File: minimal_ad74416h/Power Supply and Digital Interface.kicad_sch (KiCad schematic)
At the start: 91 parts, among them T1 ZA9644-AED, U1 MAX17570FATA+, U4 ADP1031ACPZ-2-R7, U5 ADUM1252AUA+, U6 ADUM1252AUA+, U7 ADUM1252AUA+, U8 ADUM1252AUA+

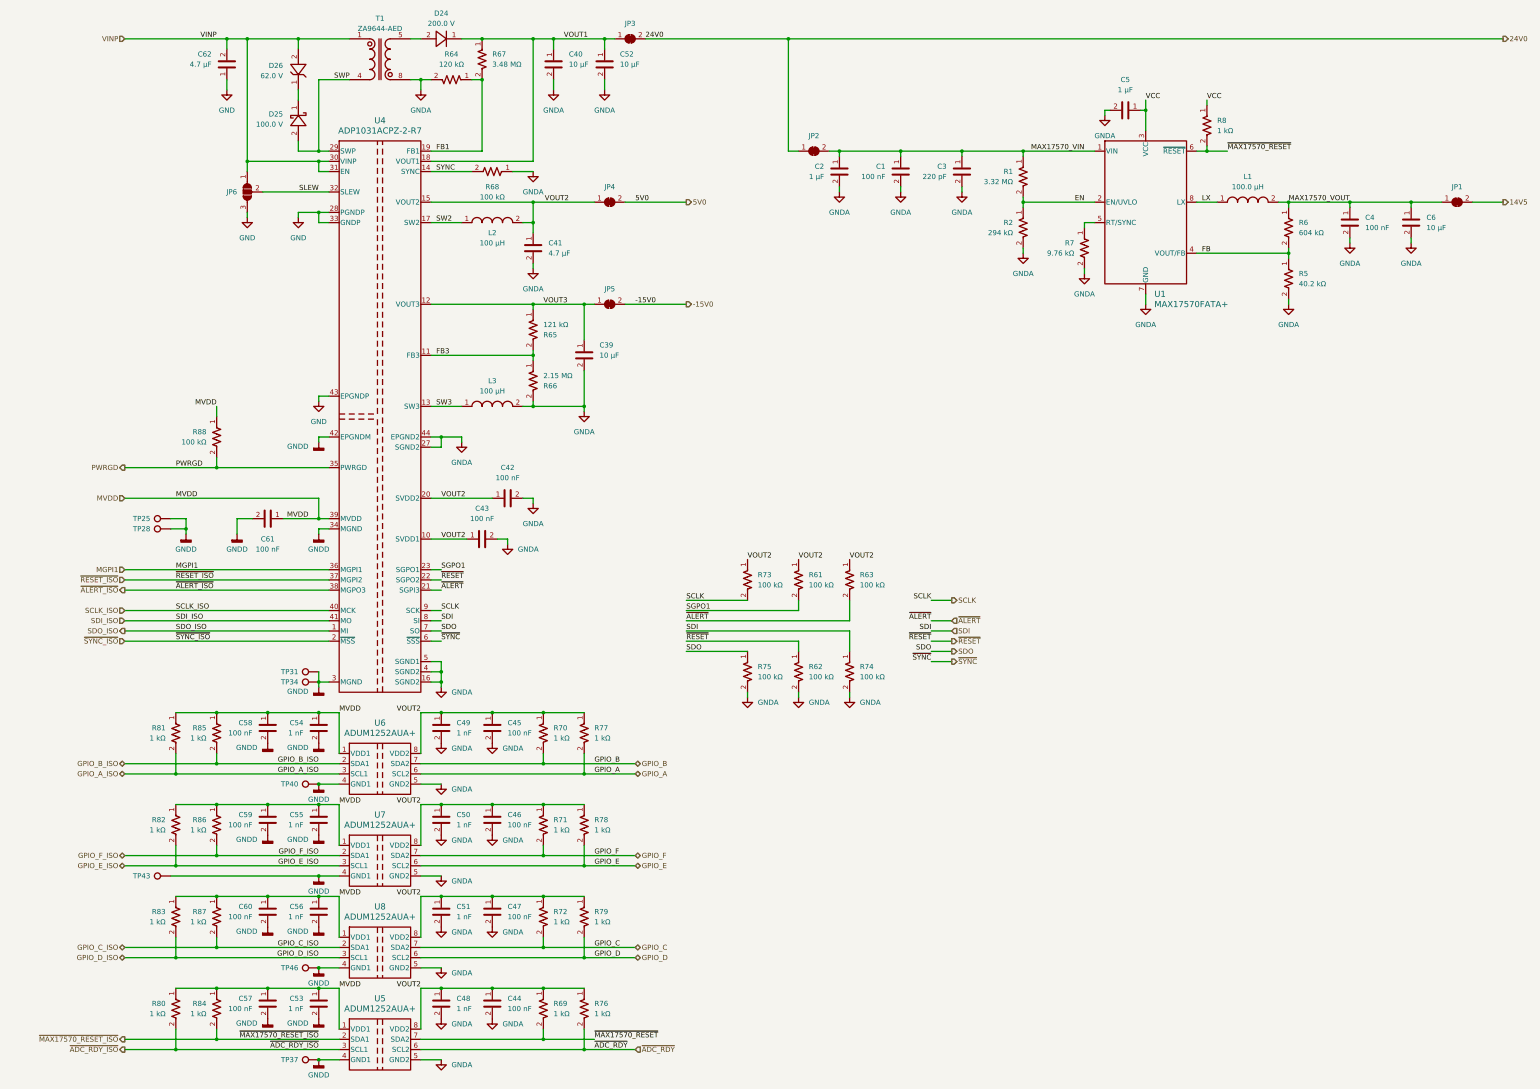
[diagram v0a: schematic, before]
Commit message: backup
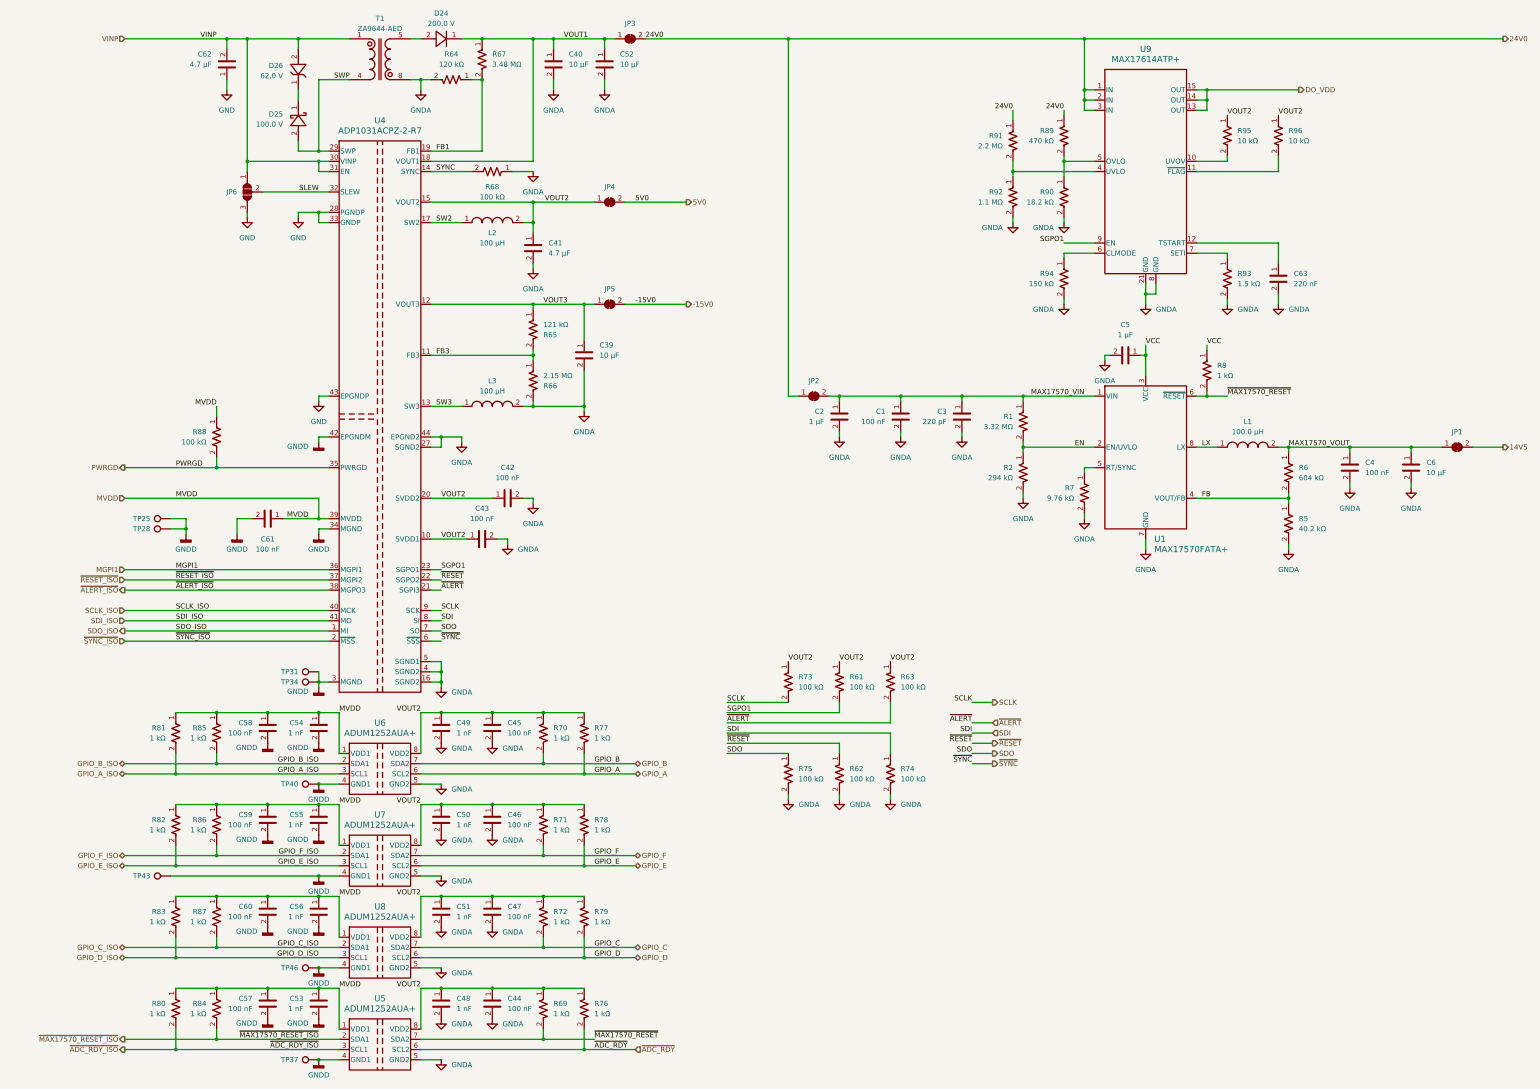
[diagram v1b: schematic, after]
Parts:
- added C63: 220 nF, capacitor_footprints:C_0402_1005Metric, symbol CAPACITORS_KGM05AR71C_DATA_BASE:C_KGM05AR71C224KH
- added R89: 470 kΩ, resistor_footprints:R_0402_1005Metric, symbol RESISTORS_RC0402FR-07_DATA_BASE:R_RC0402FR-07470KL
- added R90: 18.2 kΩ, resistor_footprints:R_0402_1005Metric, symbol RESISTORS_RC0402FR-07_DATA_BASE:R_RC0402FR-0718K2L
- added R91: 2.2 MΩ, resistor_footprints:R_0402_1005Metric, symbol RESISTORS_RC0402FR-07_DATA_BASE:R_RC0402FR-072M2L
- added R92: 1.1 MΩ, resistor_footprints:R_0402_1005Metric, symbol RESISTORS_RC0402FR-7W_DATA_BASE:R_RC0402FR-7W1M1L
- added R93: 1.5 kΩ, resistor_footprints:R_0402_1005Metric, symbol RESISTORS_ERJ-2GEJ_DATA_BASE:R_ERJ-2GEJ152X
- added R94: 150 kΩ, resistor_footprints:R_0402_1005Metric, symbol RESISTORS_ERJ-2GEJ_DATA_BASE:R_ERJ-2GEJ154X
- added R95, R96: 10 kΩ, resistor_footprints:R_0402_1005Metric, symbol UNITED_RESISTORS_DATA_BASE:R_ERJ-2RKF1002X
- added U9: MAX17614ATP+, analog_devices_footprints:21-100172_T2044&plus_4C_MXM_ADI, symbol UNITED_IC_ADI:U_MAX17614ATP+
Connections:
- net 24V0: now also R89.1, R91.1, U9.1 (IN), U9.2 (IN), U9.3 (IN)
- net GNDA: now also C63.2, R90.2, R92.2, R93.2, R94.2, U9.21 (GND), U9.8 (GND)
- net SGPO1: now also U9.9 (EN)
- net VOUT2: now also R95.1, R96.1
- new net: R96.2, U9.11 (~{FLAG})
- new net: R93.1, U9.7 (SETI)
- new net: R94.1, U9.6 (CLMODE)
- new net: C63.1, U9.12 (TSTART)
- new net: R89.2, R90.1, U9.5 (OVLO)
- new net: R95.2, U9.10 (UVOV)
- new net: R91.2, R92.1, U9.4 (UVLO)
- new net DO_VDD: U9.13 (OUT), U9.14 (OUT), U9.15 (OUT)
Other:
- moved on the sheet: C1, C2, C3, C4, C5, C6, JP1, JP2, L1, R1, R2, R5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
